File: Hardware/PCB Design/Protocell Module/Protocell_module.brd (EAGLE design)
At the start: 64.8 x 23.5 mm, 17 parts, among them IC1 MC7805BDTRKG, X3 RJ45-8X

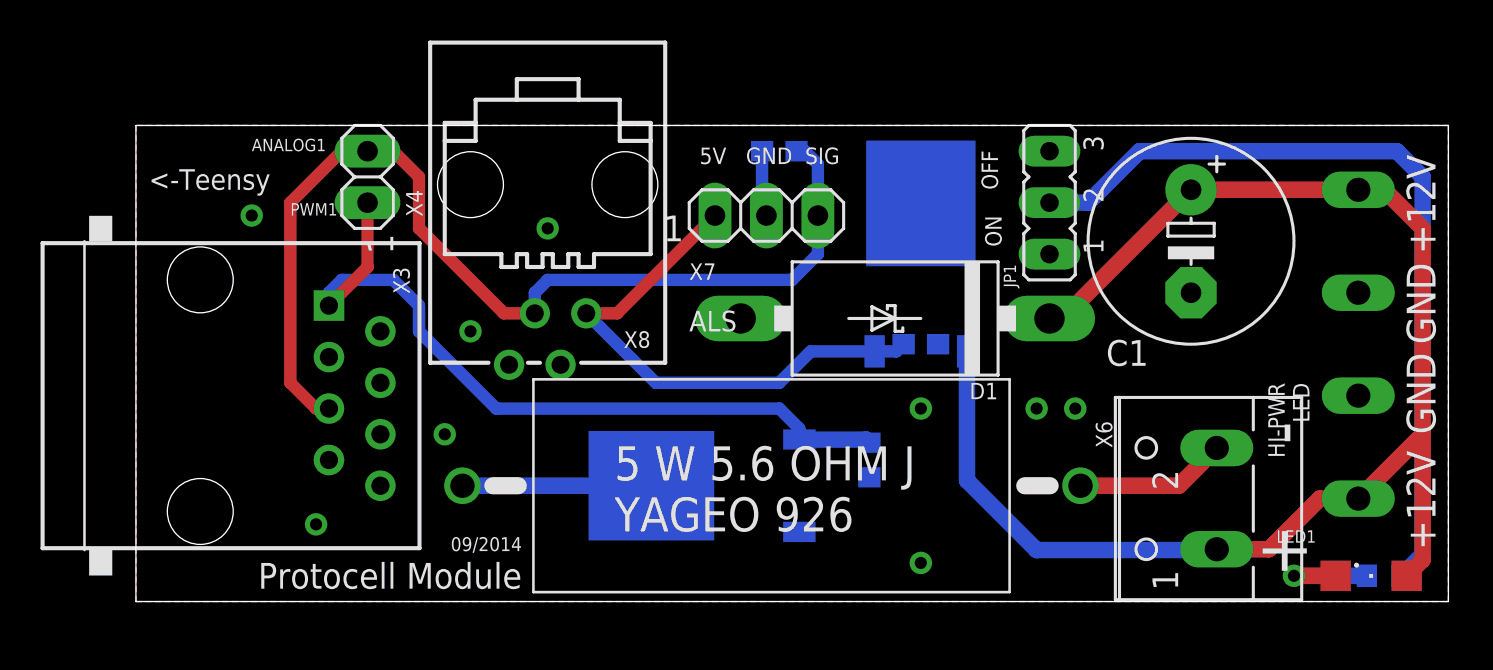
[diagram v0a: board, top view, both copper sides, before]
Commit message: Updated the board design
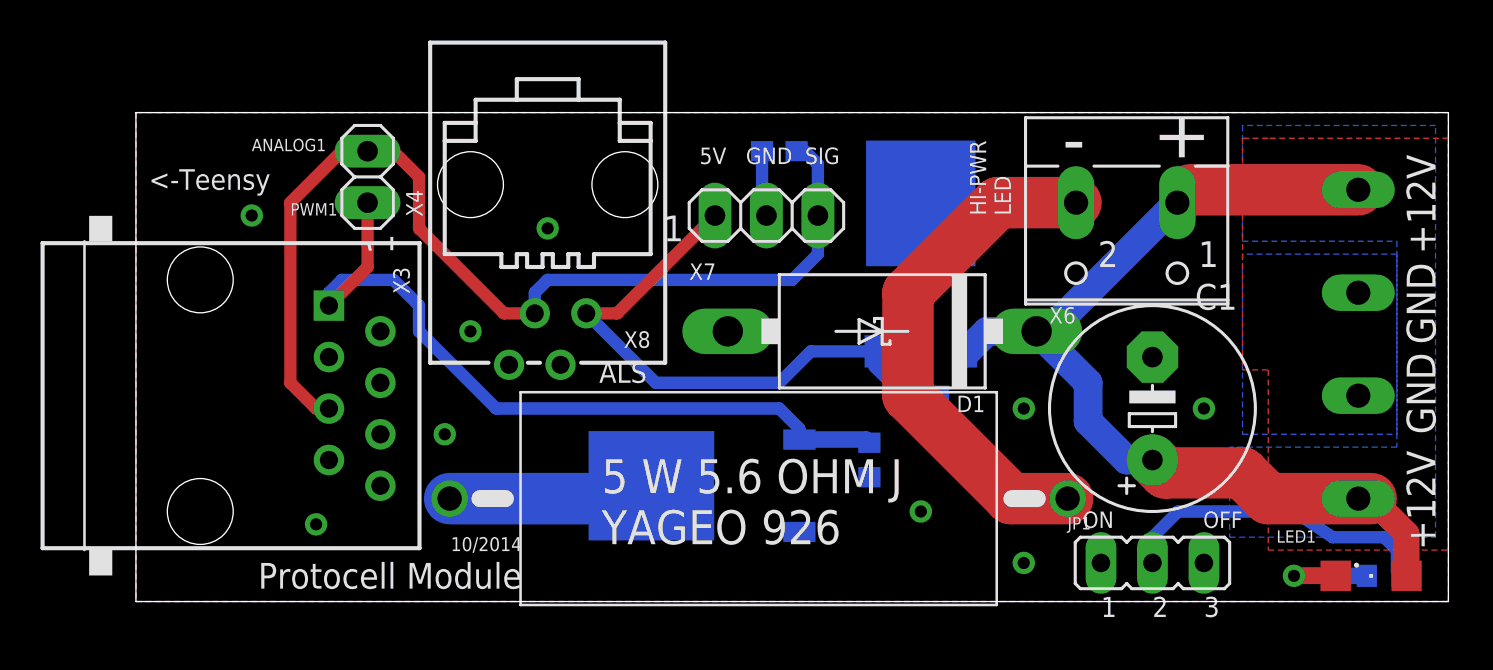
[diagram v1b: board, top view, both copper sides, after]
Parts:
- moved JP1 18.5 mm to (50.2, 1.91), turned to 0 degrees
- moved X6 13.7 mm to (48.9, 18.4), turned to 180 degrees
- moved C1 8.47 mm to (50.2, 9.53), turned to 90 degrees
- moved C2 2.54 mm to (38.7, 10.2)
- moved D1 0.90 mm to (36.8, 13.3)
- moved R3 0.90 mm to (30.5, 5.08)
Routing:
- net +12V: track 72.0 -> 47.3 mm
- net PWR_LED_GND: track 40.1 -> 15.9 mm
- net N$3: track 7.50 -> 25.2 mm
- net N$1: track 9.33 -> 10.6 mm
- net +5V: track 26.2 -> 27.4 mm
- added copper zone on layer 1, net +12V
- added copper zone on layer 16, net +12V
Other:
- board size 64.8 x 23.5 mm -> 64.8 x 24.1 mm
- board text added: "10/2014"
- board text added: "by PBAI & UWaterloo"
- board text removed: "09/2014"
